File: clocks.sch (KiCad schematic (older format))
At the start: 13 parts, among them J9 UPDI TTL, U10 ATtiny1614-SS, U11 5M1270ZT144C5N, U14 Si5351A-B-GT, X1 CB3LV-3I-100M0000, Y1 25MHZ 8PF

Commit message: parts placement
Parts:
- U10: Description (none) -> 8-bit Microcontrollers - MCU 20MHZ SOIC 85C GRN; MFR (none) -> Microchip Technology; MPN (none) -> ATTINY1614-SSNR; SPN (none) -> 556-ATTINY1614SSNR; SPR (none) -> Mouser; SPURL (none) -> https://www.mouser.com/ProductDetail/556-ATTINY1614SSNR
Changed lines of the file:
@@
 F 2 "Package_SO:SOIC-14_3.9x8.7mm_P1.27mm" H 2150 4660 50  0001 C CIN
 F 3 "http://ww1.microchip.com/downloads/en/DeviceDoc/ATtiny1614-data-sheet-40001995A.pdf" H 2150 4660 50  0001 C CNN
+F 4 "8-bit Microcontrollers - MCU 20MHZ SOIC 85C GRN" H 2150 4660 50  0001 C CNN "Description"
+F 5 "Microchip Technology" H 2150 4660 50  0001 C CNN "MFR"
+F 6 "ATTINY1614-SSNR" H 2150 4660 50  0001 C CNN "MPN"
+F 7 "556-ATTINY1614SSNR" H 2150 4660 50  0001 C CNN "SPN"
+F 8 "Mouser" H 2150 4660 50  0001 C CNN "SPR"
+F 9 "https://www.mouser.com/ProductDetail/556-ATTINY1614SSNR" H 2150 4660 50  0001 C CNN "SPURL"
 	1    2150 4660
 	1    0    0    -1

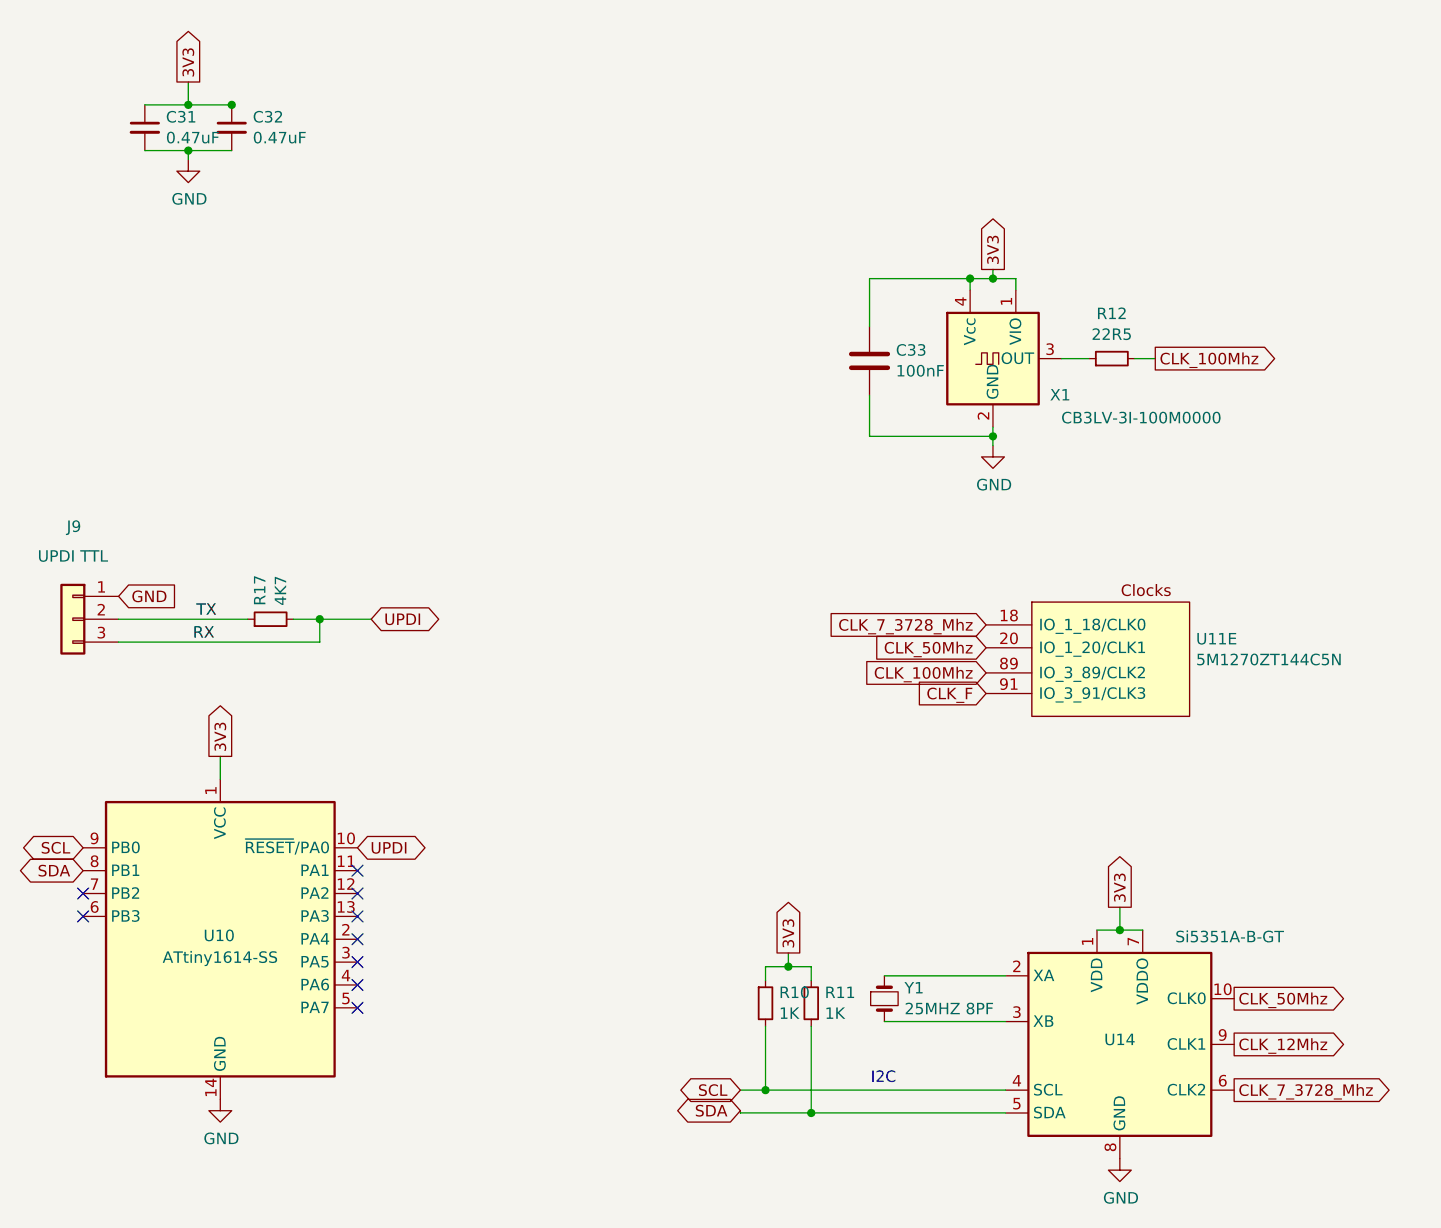
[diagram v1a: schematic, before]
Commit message: started routing
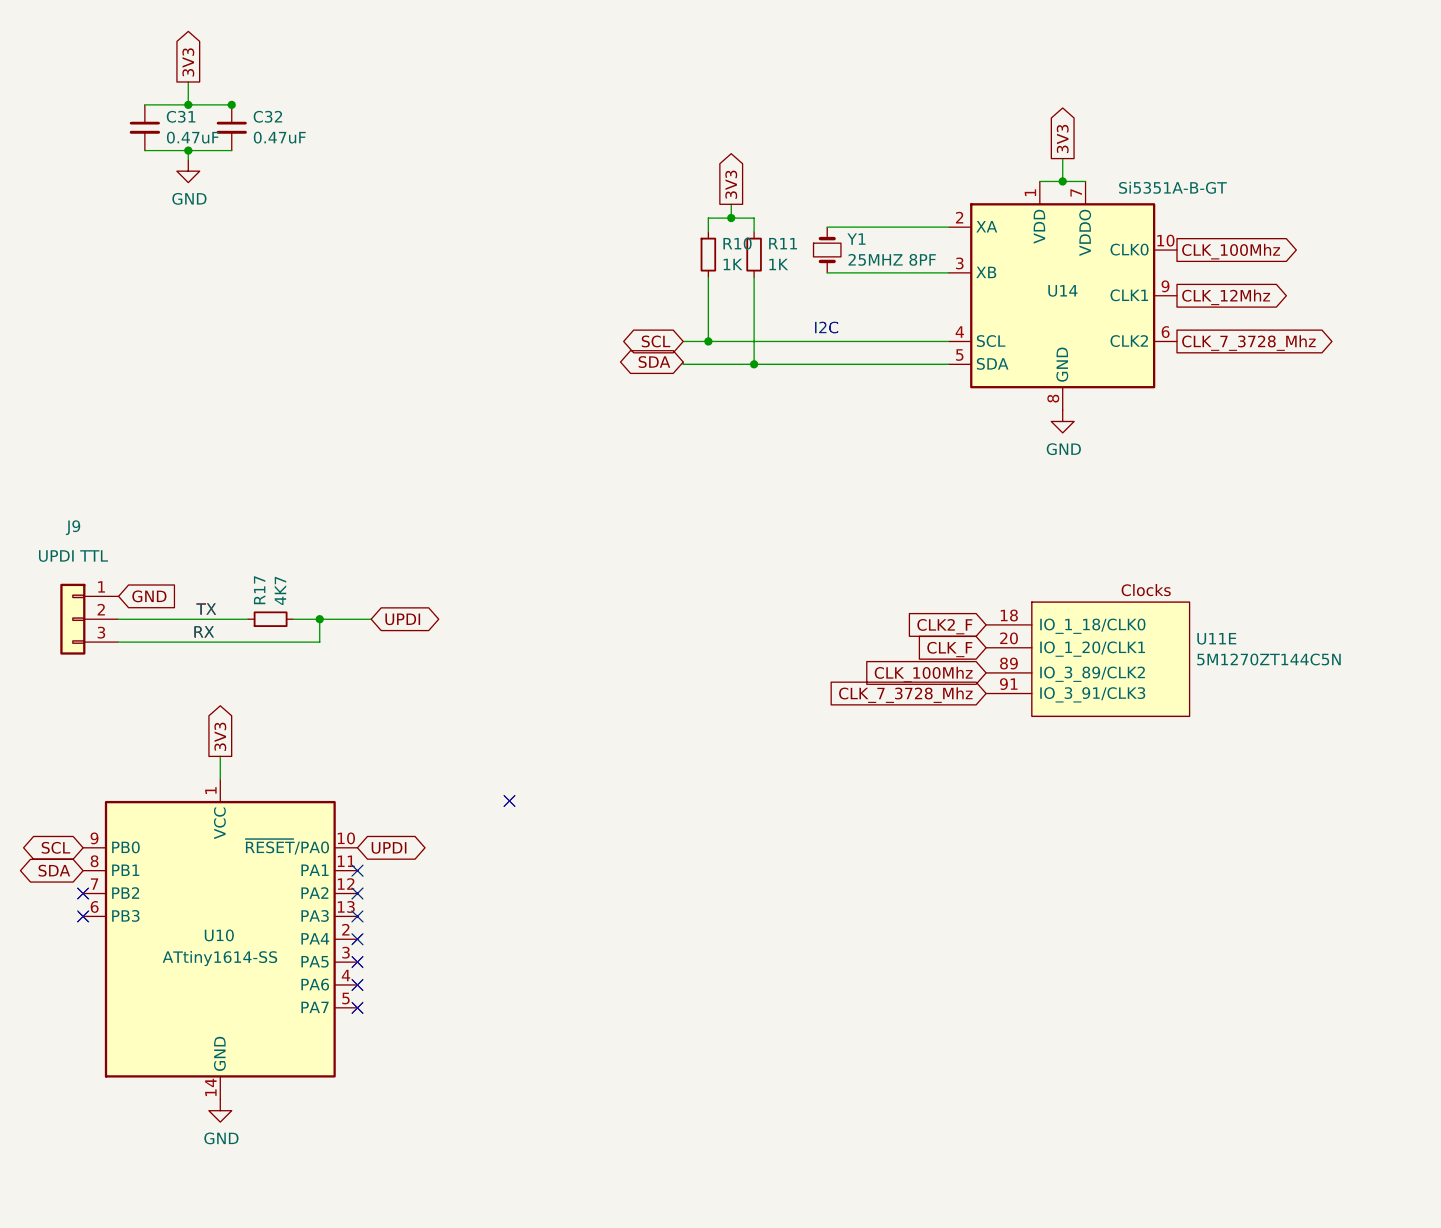
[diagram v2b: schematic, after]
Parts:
- removed C33: 100nF, Capacitor_SMD:C_0603_1608Metric_Pad1.05x0.95mm_HandSolder, symbol Device:C
- removed R12: 22R5, Resistor_SMD:R_0603_1608Metric_Pad1.05x0.95mm_HandSolder, symbol Device:R_Small
- removed X1: CB3LV-3I-100M0000, Oscillator:Oscillator_SMD_SeikoEpson_SG8002CA-4Pin_7.0x5.0mm_HandSoldering, symbol rc2014_max_v-rescue:CB3LV-3I-50M0000-Oscillator
- J9: footprint Connector_PinHeader_2.54mm:PinHeader_1x03_P2.54mm_Horizontal -> Connector_PinHeader_2.54mm:PinHeader_1x03_P2.54mm_Vertical
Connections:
- net labels added: CLK2_F
- net labels removed: CLK_50Mhz
- wire segments 43 -> 30
- no-connect marks 9 -> 10
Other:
- moved on the sheet: R10, R11, U14, Y1
